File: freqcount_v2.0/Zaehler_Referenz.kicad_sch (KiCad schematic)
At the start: 8 parts, among them U10 MCP23017_SS, U8 74AHC1G04, U9 74LV8154

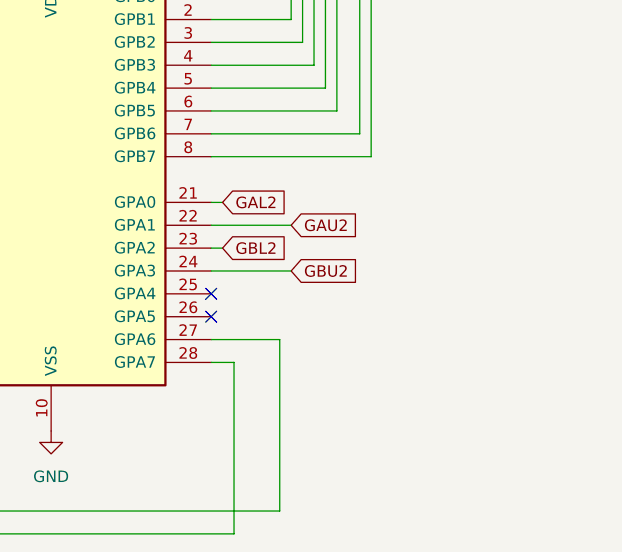
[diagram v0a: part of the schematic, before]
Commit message: update
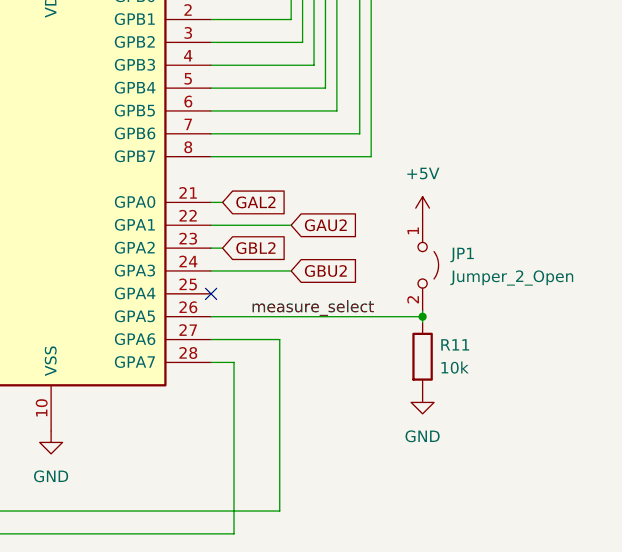
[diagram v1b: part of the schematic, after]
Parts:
- added JP1: Jumper_2_Open, Connector_PinHeader_2.54mm:PinHeader_1x02_P2.54mm_Vertical, symbol Jumper:Jumper_2_Open
- added R11: 10k, Resistor_SMD:R_0603_1608Metric, symbol Device:R
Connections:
- net +5V: now also JP1.1 (A)
- net GND: now also R11.2
- net measure_select: now reaches U10.26 (GPA5)
- net measure_select: now also JP1.2 (B), R11.1
- no-connect marks 4 -> 3
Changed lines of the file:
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@@
   (junction (at 174.625 93.98) (diameter 0) (color 0 0 0 0)
   )
+  (junction (at 233.68 106.68) (diameter 0) (color 0 0 0 0)
+  )
   (junction (at 132.715 113.03) (diameter 0) (color 0 0 0 0)
   )
@@
   (junction (at 118.745 124.46) (diameter 0) (color 0 0 0 0)
   )
-  (no_connect (at 210.185 106.68))
   (no_connect (at 174.625 88.9))
   (no_connect (at 174.625 86.36))
@@
     (stroke (width 0) (type default) (color 0 0 0 0))
   )
+  (wire (pts (xy 233.68 107.315) (xy 233.68 106.68))
+    (stroke (width 0) (type default) (color 0 0 0 0))
+  )
   (wire (pts (xy 111.125 82.55) (xy 122.555 82.55))
     (stroke (width 0) (type default) (color 0 0 0 0))
@@
     (stroke (width 0) (type default) (color 0 0 0 0))
   )
+  (wire (pts (xy 210.185 106.68) (xy 233.68 106.68))
+    (stroke (width 0) (type default) (color 0 0 0 0))
+  )
+  (wire (pts (xy 111.76 78.74) (xy 122.555 78.74))
+    (stroke (width 0) (type default) (color 0 0 0 0))
+  )
   (wire (pts (xy 145.415 45.72) (xy 219.075 45.72))
     (stroke (width 0) (type default) (color 0 0 0 0))
@@
     (stroke (width 0) (type default) (color 0 0 0 0))
   )
-  (wire (pts (xy 111.76 78.74) (xy 122.555 78.74))
-    (stroke (width 0) (type default) (color 0 0 0 0))
-  )
   (wire (pts (xy 116.205 120.65) (xy 116.205 95.25))
     (stroke (width 0) (type default) (color 0 0 0 0))
@@
     (stroke (width 0) (type default) (color 0 0 0 0))
   )
+  (wire (pts (xy 233.68 106.68) (xy 233.68 106.045))
+    (stroke (width 0) (type default) (color 0 0 0 0))
+  )
   (wire (pts (xy 83.185 120.65) (xy 94.615 120.65))
     (stroke (width 0) (type default) (color 0 0 0 0))
@@
   (wire (pts (xy 146.685 48.26) (xy 146.685 82.55))
     (stroke (width 0) (type default) (color 0 0 0 0))
+  )
+  (label "measure_select" (at 214.63 106.68 0)
+    (effects (font (size 1.27 1.27)) (justify left bottom))
   )
   (global_label "GAL2" (shape input) (at 211.455 93.98 0) (fields_autoplaced)
@@
     (pin "1")
   )
+  (symbol (lib_id "power:+5V") (at 233.68 95.885 0) (unit 1)
+    (in_bom yes) (on_board yes) (fields_autoplaced)
+    (property "Reference" "#PWR041" (id 0) (at 233.68 99.695 0)
+      (effects (font (size 1.27 1.27)) hide)
+    )
+    (property "Value" "+5V" (id 1) (at 233.68 90.805 0))
+    (property "Footprint" "" (id 2) (at 233.68 95.885 0)
+      (effects (font (size 1.27 1.27)) hide)
+    )
+    (property "Datasheet" "" (id 3) (at 233.68 95.885 0)
+      (effects (font (size 1.27 1.27)) hide)
+    )
+    (pin "1")
+  )
   (symbol (lib_id "Device:R") (at 174.625 102.87 0) (unit 1)
     (in_bom yes) (on_board yes) (fields_autoplaced)
@@
     )
     (property "Datasheet" "~" (id 3) (at 174.625 115.57 0)
+      (effects (font (size 1.27 1.27)) hide)
+    )
+    (pin "1")
+    (pin "2")
+  )
+  (symbol (lib_id "Device:R") (at 233.68 111.125 0) (unit 1)
+    (in_bom yes) (on_board yes) (fields_autoplaced)
+    (property "Reference" "R11" (id 0) (at 235.585 109.8549 0)
+      (effects (font (size 1.27 1.27)) (justify left))
+    )
+    (property "Value" "10k" (id 1) (at 235.585 112.3949 0)
+      (effects (font (size 1.27 1.27)) (justify left))
+    )
+    (property "Footprint" "Resistor_SMD:R_0603_1608Metric" (id 2) (at 231.902 111.125 90)
+      (effects (font (size 1.27 1.27)) hide)
+    )
+    (property "Datasheet" "~" (id 3) (at 233.68 111.125 0)
       (effects (font (size 1.27 1.27)) hide)
     )
@@
     (pin "9")
   )
+  (symbol (lib_id "power:GND") (at 233.68 114.935 0) (unit 1)
+    (in_bom yes) (on_board yes) (fields_autoplaced)
+    (property "Reference" "#PWR042" (id 0) (at 233.68 121.285 0)
+      (effects (font (size 1.27 1.27)) hide)
+    )
+    (property "Value" "GND" (id 1) (at 233.68 120.015 0))
+    (property "Footprint" "" (id 2) (at 233.68 114.935 0)
+      (effects (font (size 1.27 1.27)) hide)
+    )
+    (property "Datasheet" "" (id 3) (at 233.68 114.935 0)
+      (effects (font (size 1.27 1.27)) hide)
+    )
+    (pin "1")
+  )
   (symbol (lib_id "power:GND") (at 192.405 119.38 0) (unit 1)
     (in_bom yes) (on_board yes) (fields_autoplaced)
@@
     (pin "1")
   )
+  (symbol (lib_id "Jumper:Jumper_2_Open") (at 233.68 100.965 270) (unit 1)
+    (in_bom yes) (on_board yes)
+    (property "Reference" "JP1" (id 0) (at 236.855 99.6949 90)
+      (effects (font (size 1.27 1.27)) (justify left))
+    )
+    (property "Value" "Jumper_2_Open" (id 1) (at 236.855 102.2349 90)
+      (effects (font (size 1.27 1.27)) (justify left))
+    )
+    (property "Footprint" "Connector_PinHeader_2.54mm:PinHeader_1x02_P2.54mm_Vertical" (id 2) (at 233.68 100.965 0)
+      (effects (font (size 1.27 1.27)) hide)
+    )
+    (property "Datasheet" "~" (id 3) (at 233.68 100.965 0)
+      (effects (font (size 1.27 1.27)) hide)
+    )
+    (pin "1")
+    (pin "2")
+  )
   (symbol (lib_id "power:+5V") (at 132.715 72.39 0) (unit 1)
